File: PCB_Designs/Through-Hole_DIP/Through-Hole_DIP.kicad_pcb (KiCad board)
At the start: 2 copper layers, 46.9 x 22.6 mm, 13 parts, among them J1 USB-AM-S-X-X-TH, U1 ATtiny85-20P, Y1 12MHz

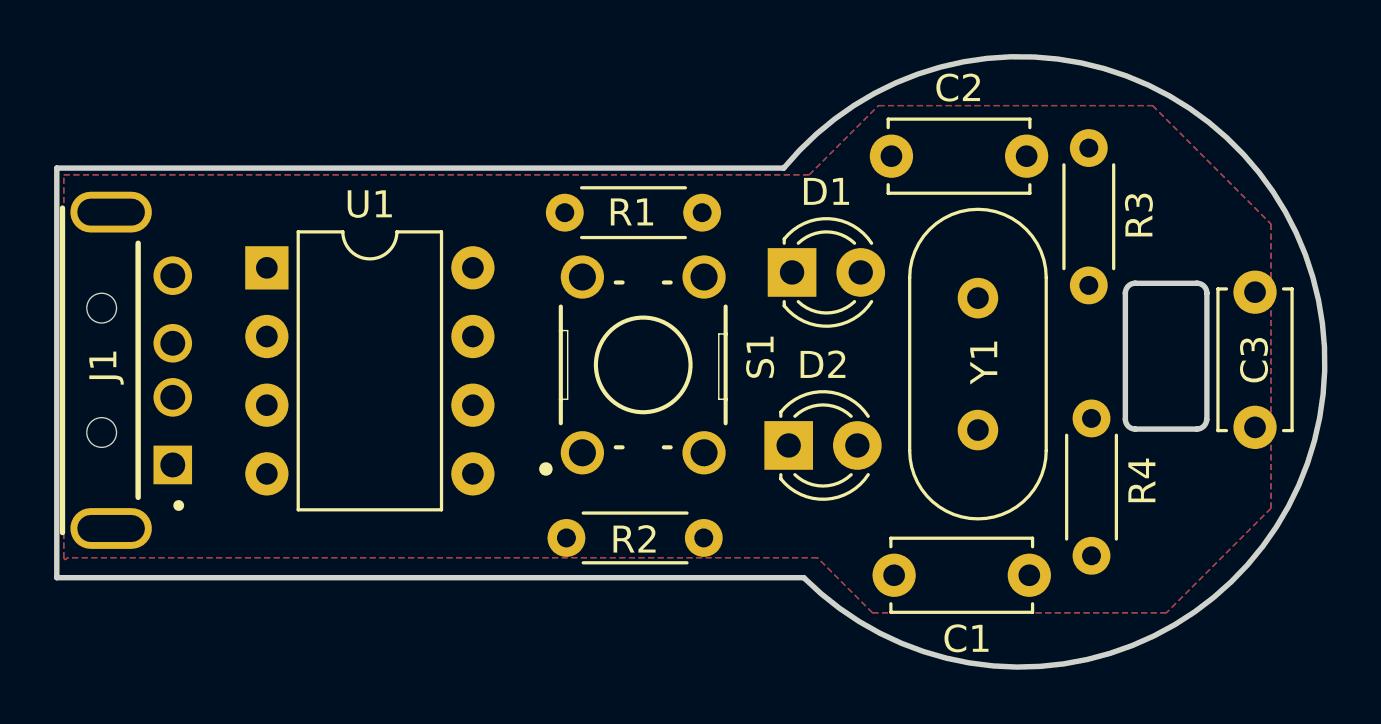
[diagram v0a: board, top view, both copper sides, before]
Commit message: Modified
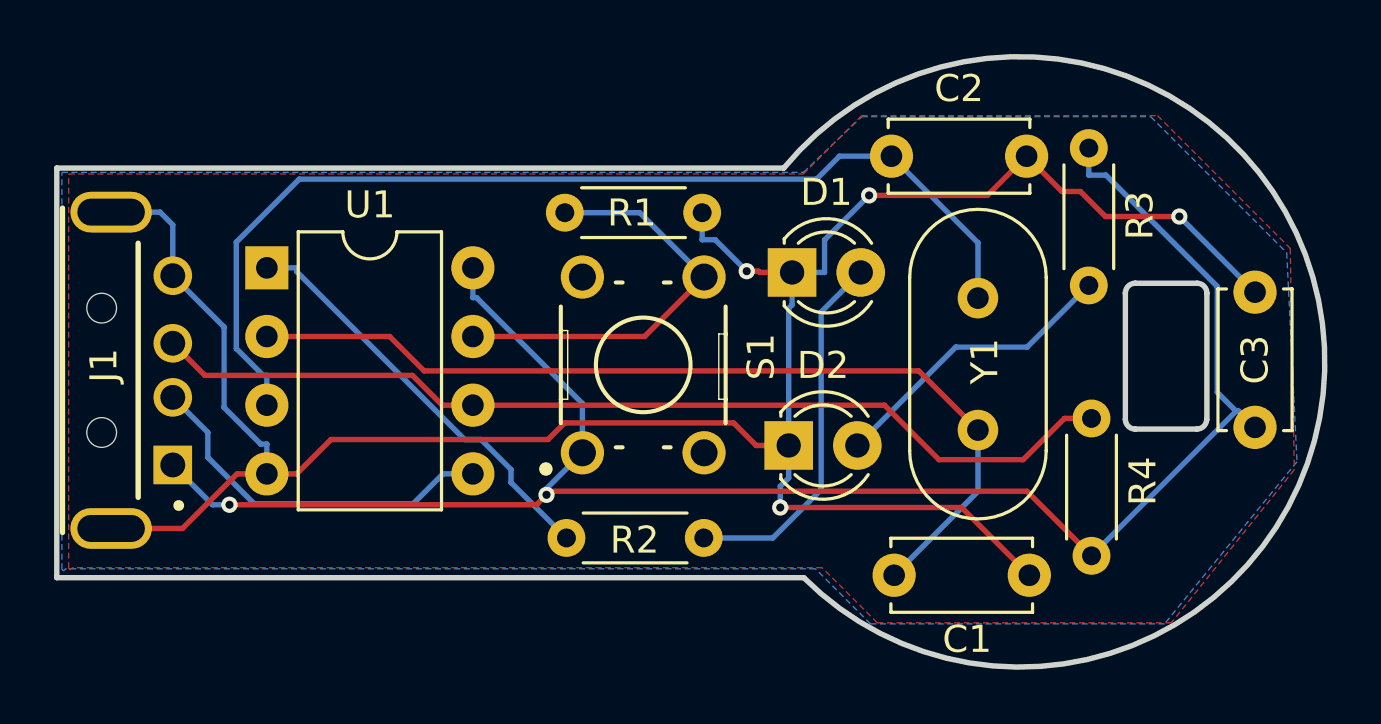
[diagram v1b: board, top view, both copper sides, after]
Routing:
- net GND: track 0.00 -> 85.9 mm, vias 0 -> 4
- net +5V: track 0.00 -> 67.4 mm, vias 0 -> 2
- net Net-(U1-XTAL2/PB4): track 0.00 -> 38.7 mm
- net /Data+: track 0.00 -> 36.4 mm
- net Net-(U1-XTAL1/PB3): track 0.00 -> 34.4 mm
- net Net-(U1-PB2): track 0.00 -> 15.6 mm
- net Net-(U1-~{RESET}/PB5): track 0.00 -> 15.6 mm
- net /Data-: track 0.00 -> 13.7 mm
- net Net-(D1-A): track 0.00 -> 13.7 mm
- net Net-(D2-A): track 0.00 -> 11.0 mm
